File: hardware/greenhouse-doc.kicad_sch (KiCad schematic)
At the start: 34 parts, among them IC1 SC810ULTRT, IC2 TPS564247DRLR, J1 USB_B_Micro, J2 Conn_02x03_Odd_Even, J3 Conn_01x02, J4 Conn_01x02, J5 Conn_01x02, K1 ADW1203HLW, Q1 2N7002, Q2 2N7002, U1 ESP32-WROOM-32, U2 DS18B20

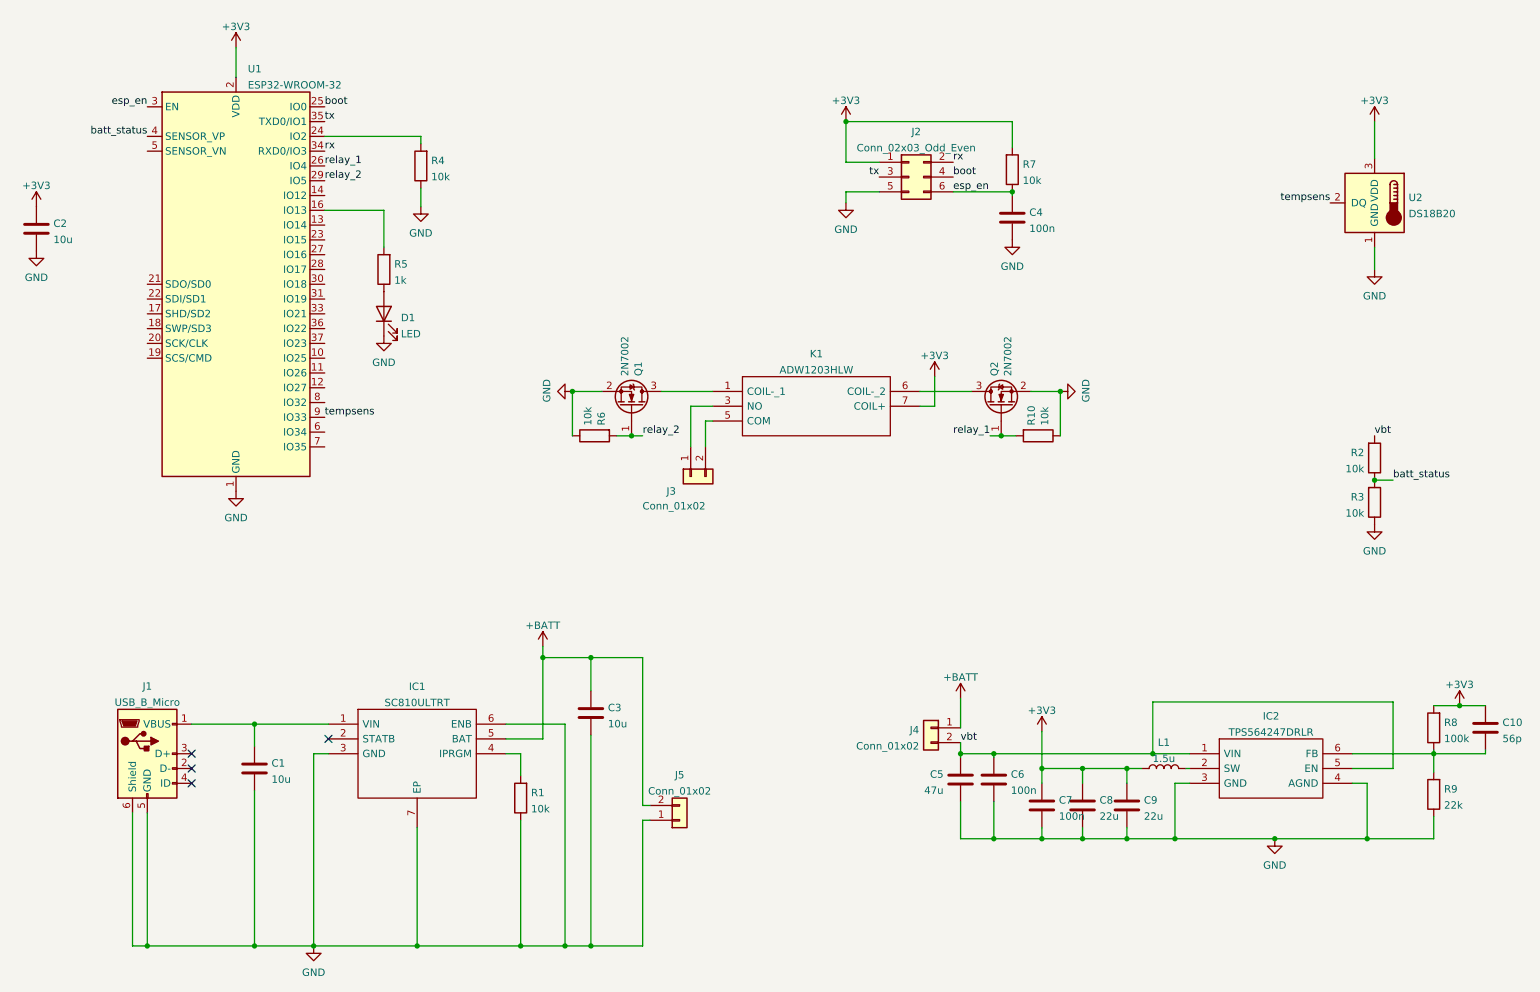
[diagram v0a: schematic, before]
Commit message: v2 hardware
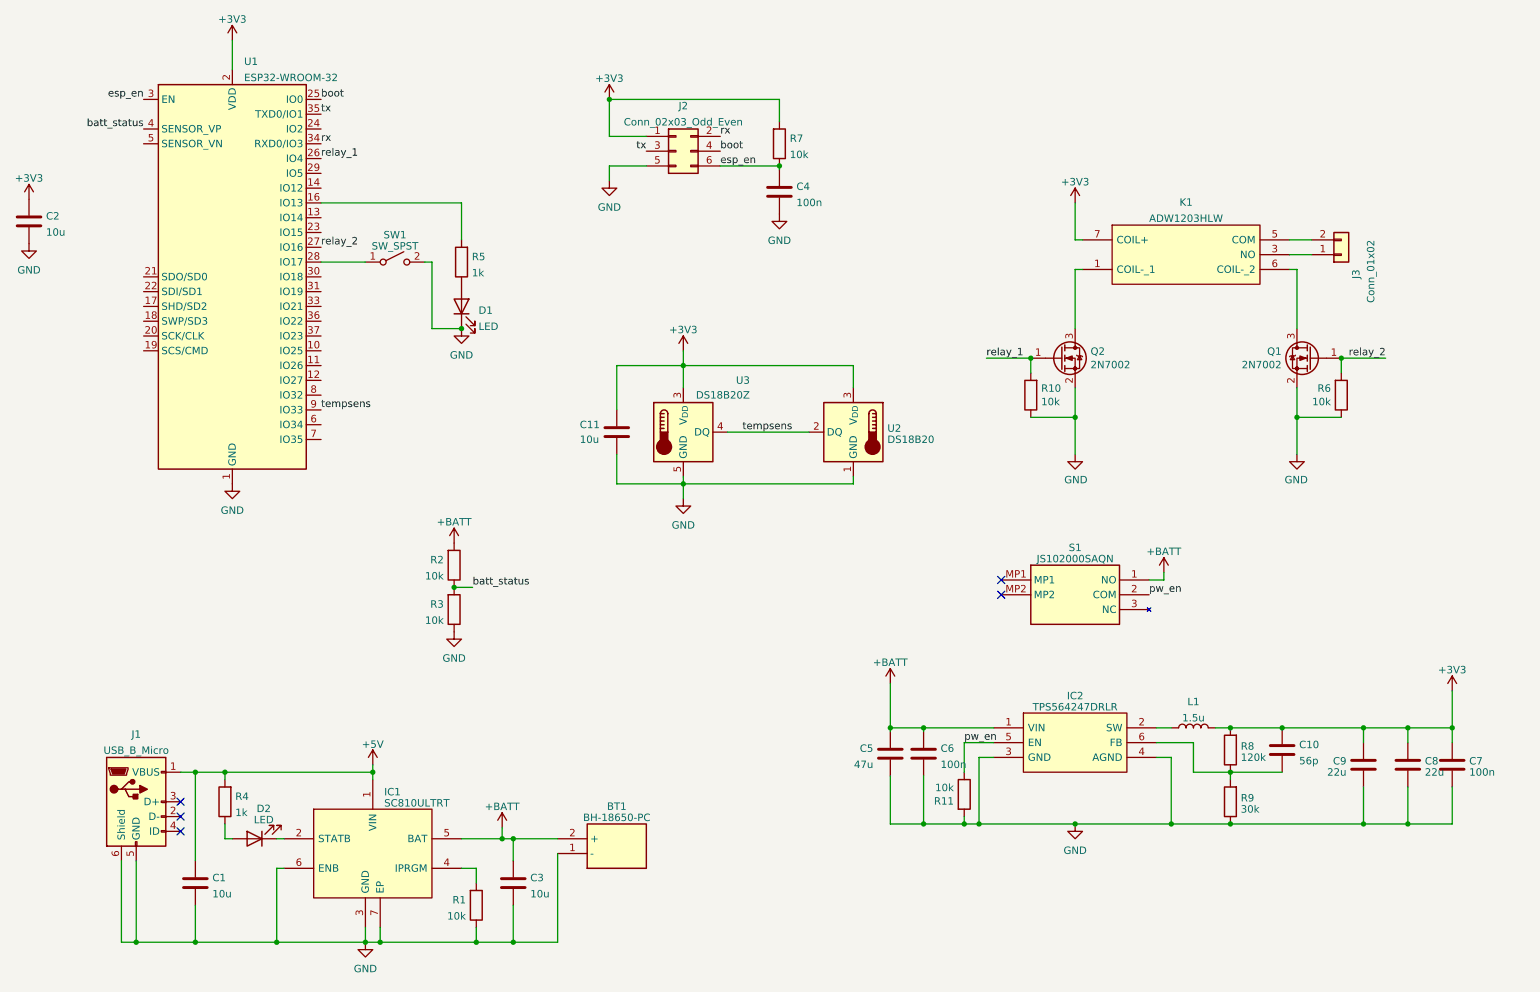
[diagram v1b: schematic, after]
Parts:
- removed J4, J5: Conn_01x02, Connector_PinHeader_2.54mm:PinHeader_1x02_P2.54mm_Vertical, symbol Connector_Generic:Conn_01x02
- added BT1: BH-18650-PC, SamacSys_Parts:BH18650PC, symbol SamacSys_Parts:BH-18650-PC
- added C11: 10u, Capacitor_SMD:C_0805_2012Metric, symbol Device:C
- added D2: LED, LED_SMD:LED_0805_2012Metric, symbol Device:LED
- added R11: 10k, Resistor_SMD:R_0805_2012Metric, symbol Device:R
- added S1: JS102000SAQN, SamacSys_Parts:JS102000SAQN, symbol SamacSys_Parts:JS102000SAQN
- added SW1: SW_SPST, Button_Switch_THT:SW_Tactile_SPST_Angled_PTS645Vx58-2LFS, symbol Switch:SW_SPST
- added U3: DS18B20Z, Package_SO:SOIC-8_3.9x4.9mm_P1.27mm, symbol Sensor_Temperature:DS18B20Z
- C1, C2, C3, C4: footprint Capacitor_SMD:C_0805_2012Metric_Pad1.18x1.45mm_HandSolder -> Capacitor_SMD:C_0805_2012Metric
- C10, C6, C7: footprint Capacitor_SMD:C_0603_1608Metric_Pad1.08x0.95mm_HandSolder -> Capacitor_SMD:C_0805_2012Metric
- R4: value 10k -> 1k
- R8: value 100k -> 120k; footprint Resistor_SMD:R_0603_1608Metric_Pad0.98x0.95mm_HandSolder -> Resistor_SMD:R_0805_2012Metric
- R9: value 22k -> 30k; footprint Resistor_SMD:R_0603_1608Metric_Pad0.98x0.95mm_HandSolder -> Resistor_SMD:R_0805_2012Metric
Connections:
- net +3V3: now also C11.1, U3.3 (V_{DD})
- net +BATT: now also C5.1, C6.1, IC2.1 (VIN), R2.2, BT1.2 (+), S1.1 (NO)
- net GND: now also BT1.1 (-), C11.2, R11.2, SW1.2 (B), U3.5 (GND); no longer R4.1
- net relay_2: now also U1.27 (IO16); no longer U1.29 (IO5)
- net tempsens: now also U3.4 (DQ)
- net at Q1.3 (D): now also K1.6 (COIL-_2); no longer K1.1 (COIL-_1)
- net at U1.24 (IO2): no longer R4.2
- net at U1.28 (IO17): now also SW1.1 (A)
- net +5V: now reaches C1.1, IC1.1 (VIN), J1.1 (VBUS)
- net +5V: now also R4.2
- net at IC1.2 (STATB): now also D2.1 (K)
- net at Q2.3 (D): now also K1.1 (COIL-_1); no longer K1.6 (COIL-_2)
- removed net vbt: C5.1, C6.1, IC2.1 (VIN), IC2.5 (EN), R2.2
- new net: D2.2 (A), R4.1
- new net pw_en: IC2.5 (EN), R11.1, S1.2 (COM)
- no-connect marks 4 -> 5
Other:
- moved on the sheet: C1, C10, C2, C3, C4, C5, C6, C7, C8, C9, D1, J1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
